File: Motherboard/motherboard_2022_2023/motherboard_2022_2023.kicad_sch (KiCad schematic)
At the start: 16 parts, among them J1 Conn_01x02_Female, J10 Conn_01x03_Male, J2 Raspberry_Pi_2_3, J3 Conn_01x03_Male, J4 Conn_01x03_Male, J5 Conn_01x03_Male, J6 Conn_01x03_Male, J7 Conn_01x03_Male, J8 Conn_01x03_Male, J9 Conn_01x03_Male, U1 XBee_THT, U2 BNO055, U3 PCA9685PW, U4 MPL3115A2

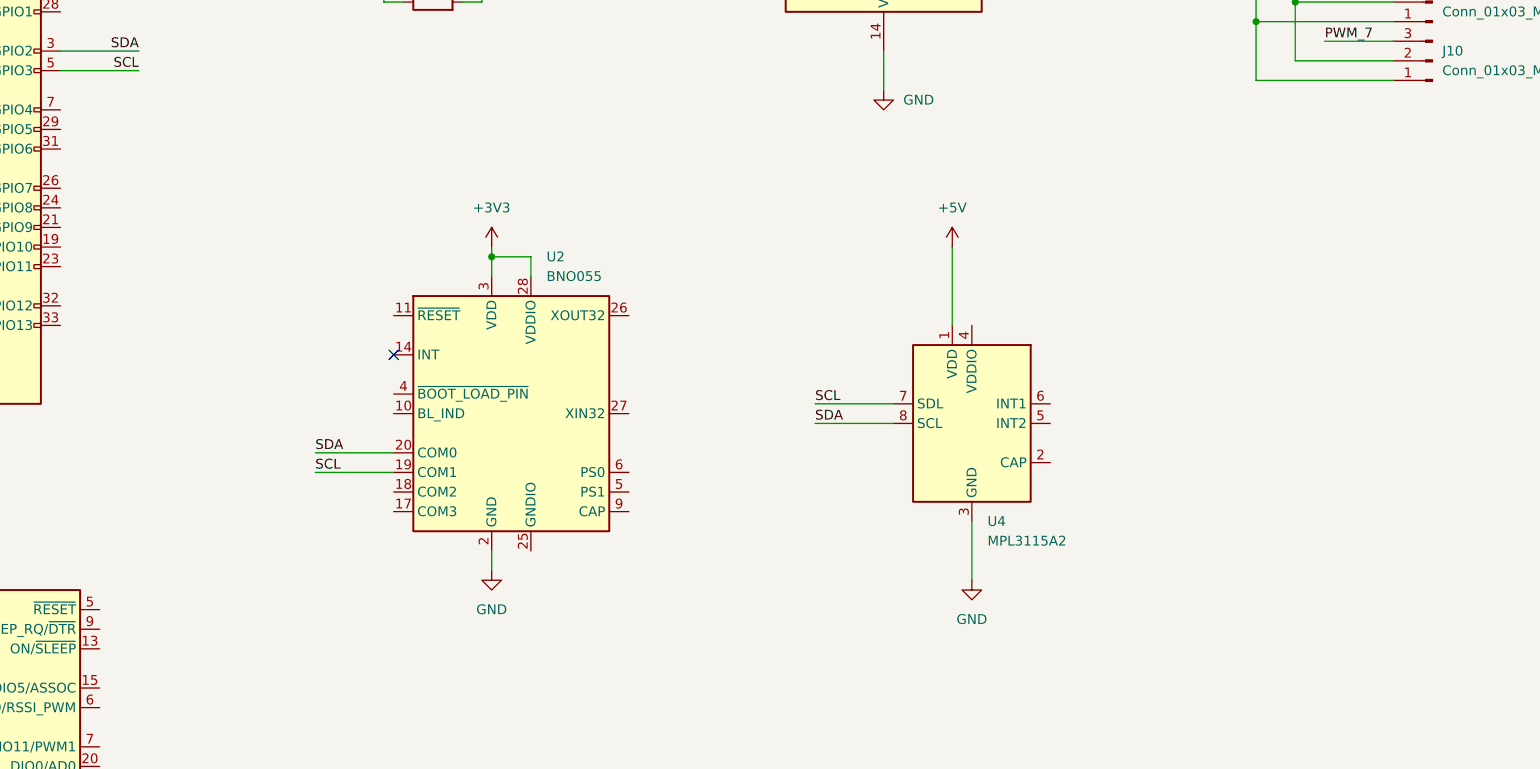
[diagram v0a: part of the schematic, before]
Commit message: Add SAM-M8Q
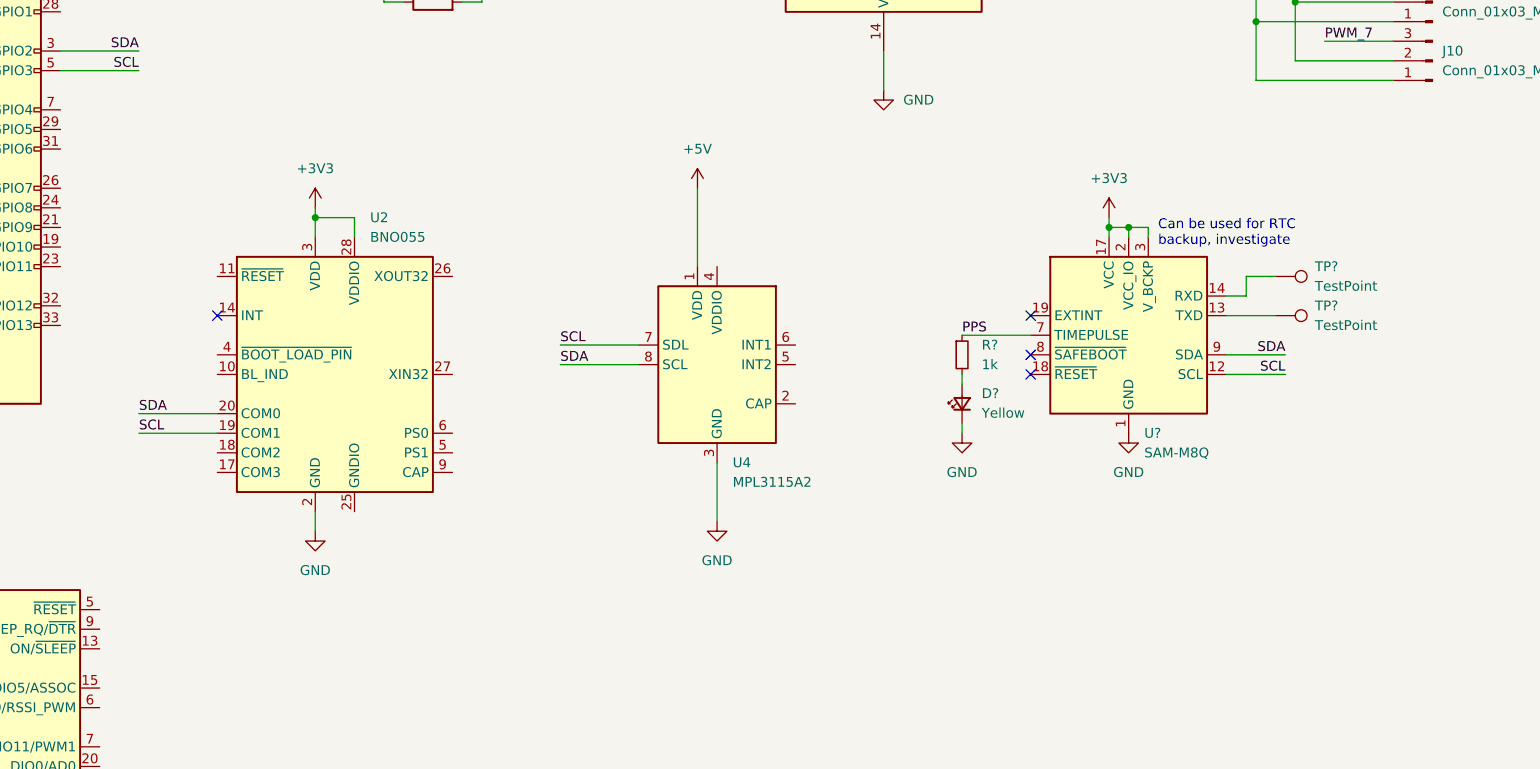
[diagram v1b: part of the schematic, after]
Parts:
- added D?: Yellow, symbol Device:LED_Small
- added R?: 1k, symbol Device:R_Small
- added TP? (x2): TestPoint, symbol Connector:TestPoint
- added U?: SAM-M8Q, RF_GPS:ublox_SAM-M8Q, symbol RF_GPS:SAM-M8Q
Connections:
- net +3V3: now also U?.17 (VCC), U?.2 (VCC_IO), U?.3 (V_BCKP)
- net GND: now also D?.1 (K), U?.1 (GND), U?.10 (GND), U?.11 (GND), U?.15 (GND), U?.16 (GND), U?.20 (GND), U?.4 (GND), U?.5 (GND), U?.6 (GND)
- net SCL: now also U?.12 (SCL)
- net SDA: now also U?.9 (SDA)
- new net: TP?.1, U?.13 (TXD)
- new net: TP?.1, U?.14 (RXD)
- new net: D?.2 (A), R?.2
- new net PPS: R?.1, U?.7 (TIMEPULSE)
- no-connect marks 8 -> 11
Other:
- note added: "Can be used for RTC backup, investigate"
- moved on the sheet: U2, U4
